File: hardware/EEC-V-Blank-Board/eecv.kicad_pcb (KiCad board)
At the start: 2 copper layers, 140.8 x 164.4 mm, 1 part, among them J1 EEC-V

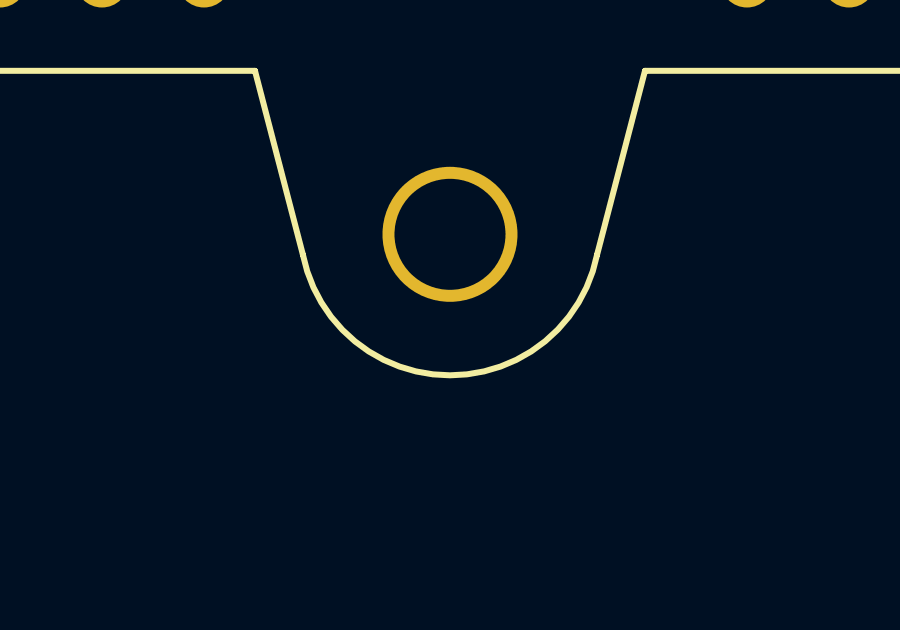
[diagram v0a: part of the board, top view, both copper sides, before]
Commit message: update pcb files
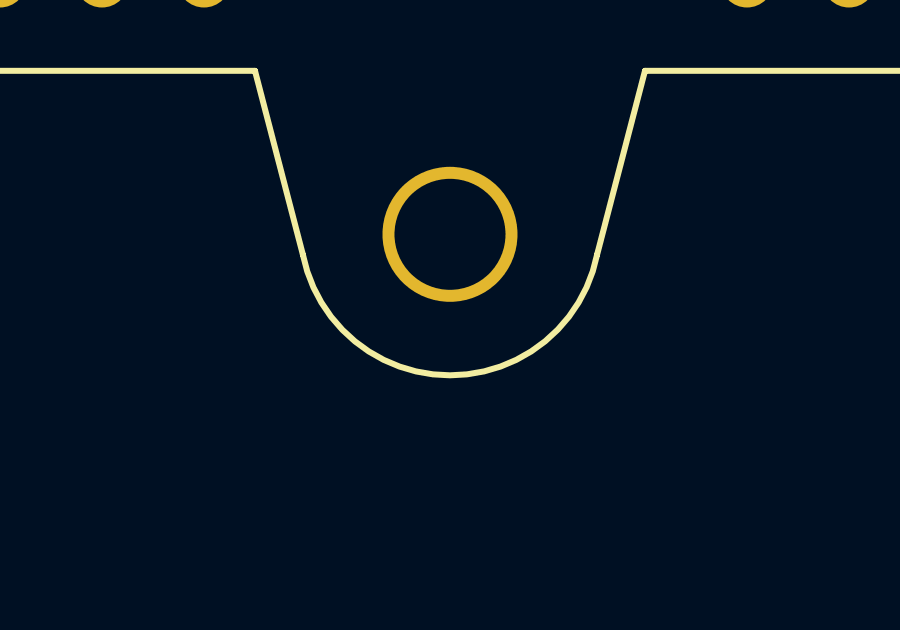
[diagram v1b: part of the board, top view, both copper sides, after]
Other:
- net class Default removed
